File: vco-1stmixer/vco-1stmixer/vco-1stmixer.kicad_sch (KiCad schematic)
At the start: 48 parts, among them J101 VCO Control In, J102 1st IF Out, J103 VCO Sample, J104 RF In, J105 Conn_01x02, U101 POS-200, U102 MAV-11, U103 MAV-11, U104 TUF-1H+

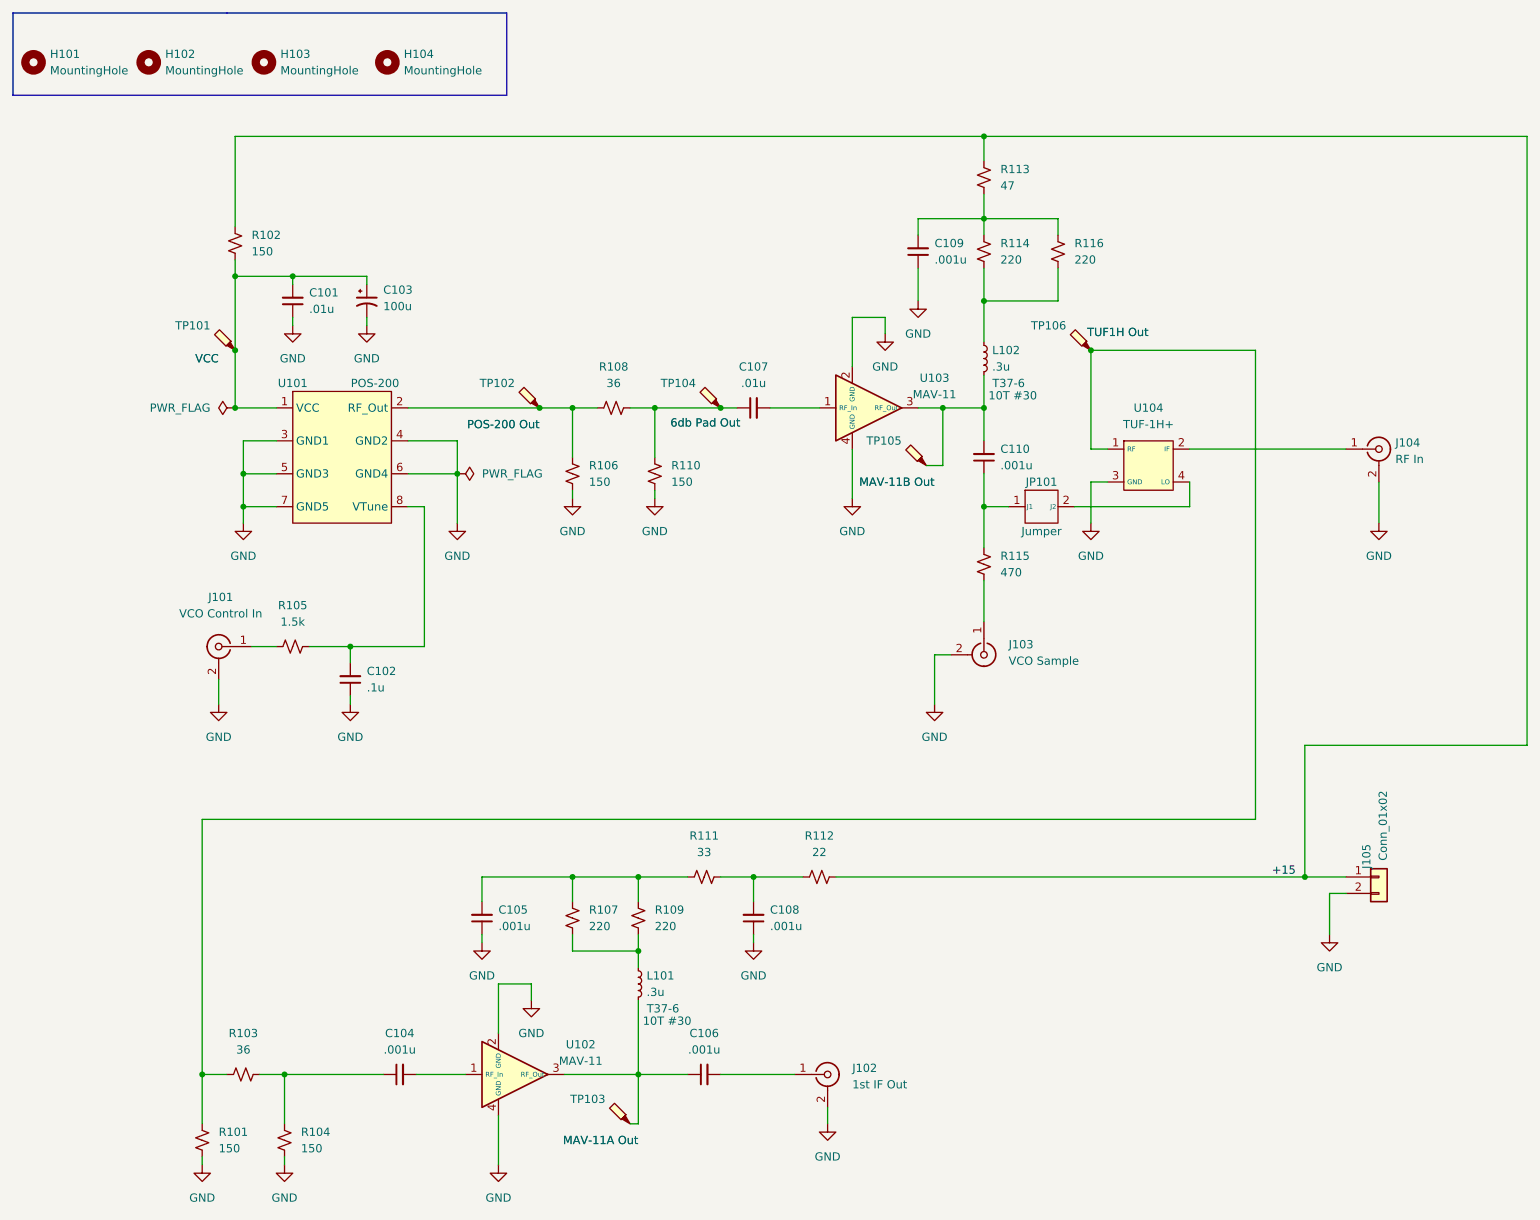
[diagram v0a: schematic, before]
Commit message: 1st mixer VCO pcb rev 2
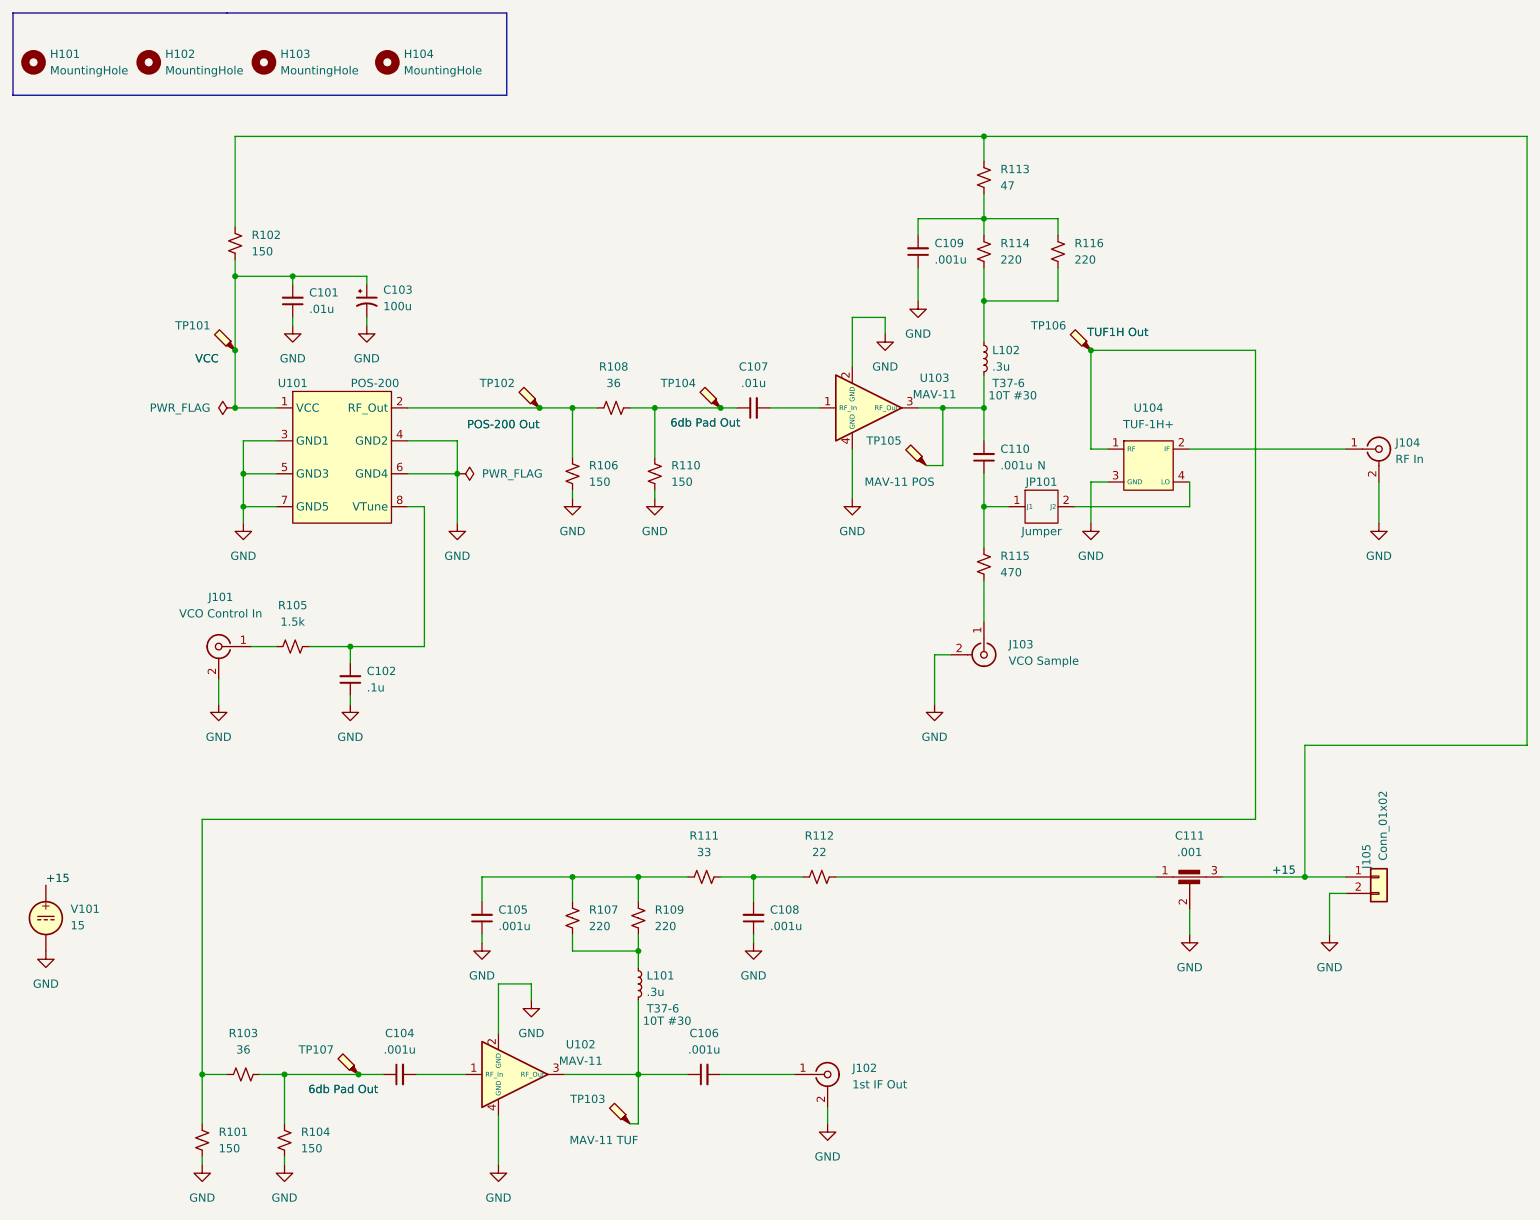
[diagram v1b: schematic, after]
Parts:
- added C111: .001, spectrum-analyzer:DSS1N_MUR, symbol Device:C_Feedthrough
- added TP107: ${SIM.PARAMS}, TestPoint:TestPoint_Pad_1.0x1.0mm, symbol Connector:TestPoint_Probe
- added V101: 15, symbol Simulation_SPICE:VDC
- J103: footprint Connector_Wire:SolderWire-0.5sqmm_1x02_P4.6mm_D0.9mm_OD2.1mm -> Connector_PinHeader_2.54mm:PinHeader_1x02_P2.54mm_Vertical
- J105: footprint vco-1stmixer:691103110002 -> Connector_Wire:SolderWire-0.5sqmm_1x02_P4.6mm_D0.9mm_OD2.1mm
- JP101: Spice_Netlist_Enabled (none) -> N
- TP102: value ${SIM.PARAMS} -> POS-200 Out
- TP103: value ${SIM.PARAMS} -> MAV-11 TUF
- TP105: value ${SIM.PARAMS} -> MAV-11 POS
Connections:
- net +15: now also C111.3, V101.1; no longer R112.2
- net GND: now also C111.2, V101.2
- net at C104.1, R103.2, R104.2: now also TP107.1
- new net: C111.1, R112.2
